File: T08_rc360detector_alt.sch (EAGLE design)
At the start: 53 parts, among them IC1 LM317MSTT3, IC2 LM317MSTT3, IC3 LM1117, U2 ATMEGA328P_PDIP, X1 SSW-101-02-S-D, X3 SSW-101-02-S-D, X4 87758-0616, X5 87758-0616, X6 SSW-104-02-S-Q

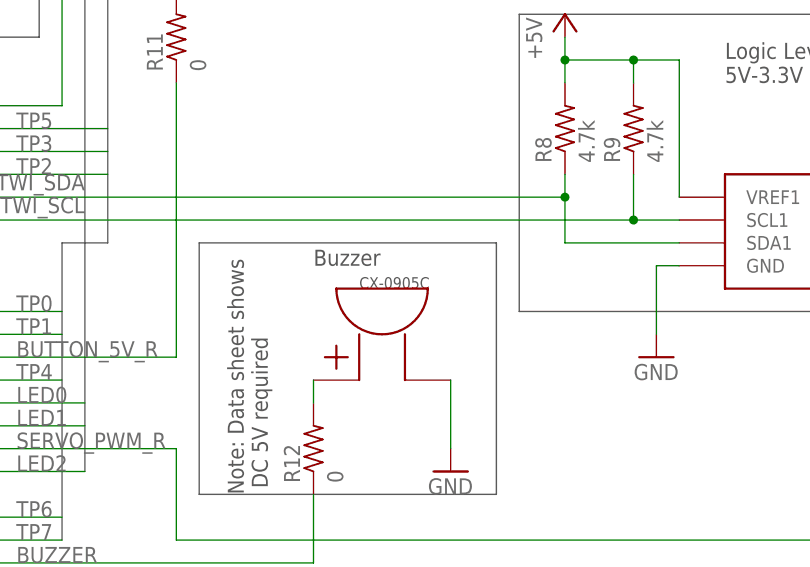
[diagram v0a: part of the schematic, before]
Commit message: Slight changes. Passed DRC
Made sure DRC worked and had updated libraries. This should work now,
(hopefully)
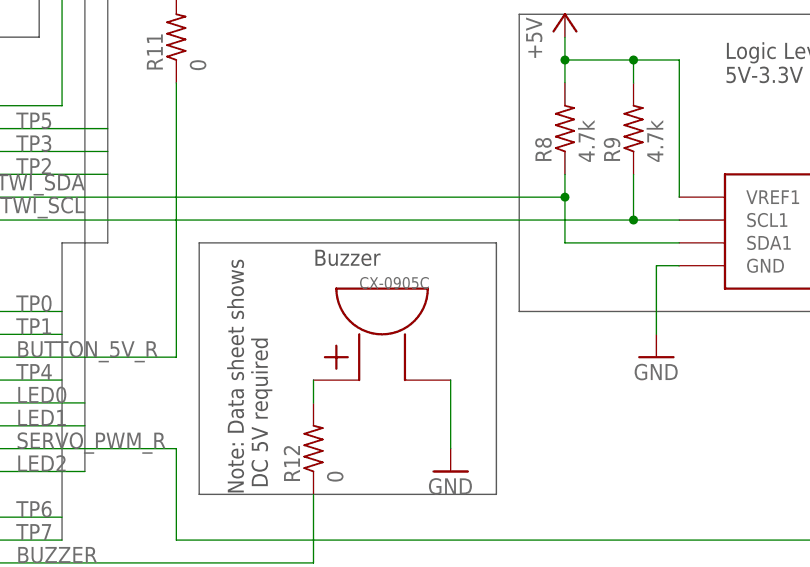
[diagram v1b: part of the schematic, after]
